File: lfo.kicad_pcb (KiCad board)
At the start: 2 copper layers, 103.7 x 33.7 mm, 34 parts, among them J1 PJ398SM-12 (Tri), J2 PJ398SM-12 (square), J3 PJ398SM-12 (weird), J4 Conn_02x05_Odd_Even, Q1 BC547, SW1 SW_SPDT, U1 TL084

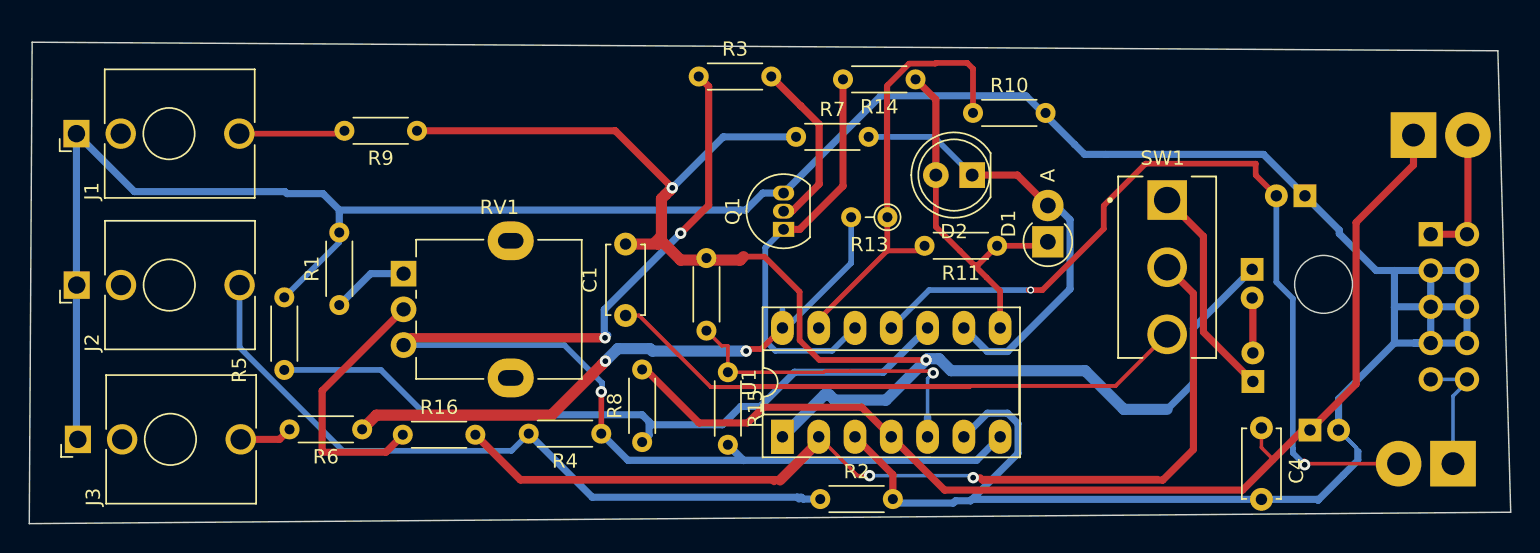
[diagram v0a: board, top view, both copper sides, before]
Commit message: base commit
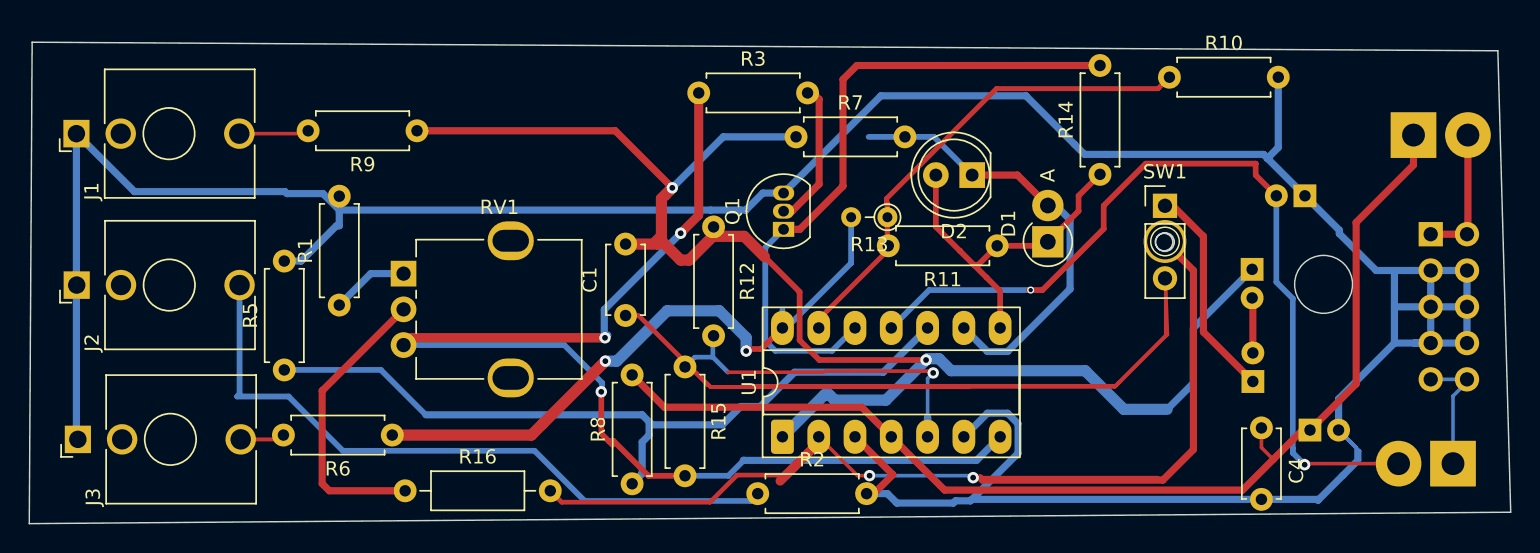
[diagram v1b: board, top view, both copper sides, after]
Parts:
- removed R4: 2.2kR, Resistor_THT:R_Axial_DIN0204_L3.6mm_D1.6mm_P5.08mm_Horizontal
- R1, R10, R11, R12, R14, R15, R2, R3, R5, R6, R7, R8, R9: footprint Resistor_THT:R_Axial_DIN0204_L3.6mm_D1.6mm_P5.08mm_Horizontal -> Resistor_THT:R_Axial_DIN0207_L6.3mm_D2.5mm_P7.62mm_Horizontal
- R16: footprint Resistor_THT:R_Axial_DIN0204_L3.6mm_D1.6mm_P5.08mm_Horizontal -> Resistor_THT:R_Axial_DIN0207_L6.3mm_D2.5mm_P10.16mm_Horizontal
- SW1: footprint 100SP1T1B4M2QE:SW_100SP1T1B4M2QE -> Connector_PinHeader_2.54mm:PinHeader_1x03_P2.54mm_Vertical
- moved R14 14.5 mm to (131.8, 20.4), turned to 90 degrees
- moved R10 14.0 mm to (136.7, 13.6)
- moved R2 4.40 mm to (107.9, 42.7)
- moved SW1 4.30 mm to (136.4, 22.6)
- moved R16 3.93 mm to (83.2, 42.5)
- moved R15 3.02 mm to (102.8, 33.8)
- moved R8 3.00 mm to (99.1, 42.0)
- moved R12 2.24 mm to (104.8, 24.0)
- moved R6 2.15 mm to (82.3, 38.6)
- moved R3 1.15 mm to (103.8, 14.7)
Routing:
- net Net-(SW1-C): track 75.2 -> 119.7 mm
- net Net-(SW1-B): track 108.0 -> 78.8 mm
- net Net-(R15-Pad2): track 109.4 -> 83.7 mm
- net Net-(Q1-C): track 28.5 -> 46.8 mm
- net Net-(U1D--): track 45.4 -> 34.4 mm
- net GND: track 234.7 -> 241.6 mm
- net Net-(U1C-+): track 51.1 -> 54.3 mm
- net Net-(J2-PadT): track 50.6 -> 47.6 mm
- net Net-(J1-PadT): track 7.44 -> 4.90 mm
- net Net-(R16-Pad1): track 18.5 -> 20.6 mm
- net Net-(Q1-B): track 12.2 -> 10.2 mm
- net Net-(C1-Pad2): track 106.9 -> 108.1 mm
- net Net-(D1-K): track 25.7 -> 24.6 mm
- net Net-(R13-Pad2): track 43.7 -> 44.5 mm
- net Net-(U1B-+): track 24.4 -> 25.2 mm
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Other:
- outline, holes or cut-outs redrawn
